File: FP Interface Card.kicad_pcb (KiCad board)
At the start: 6 copper layers, 90.2 x 101.1 mm, 274 parts, among them J1 T1M-10-F-SV-L, J2 T1M-10-F-SV-L, J3 ZX62-AB-5PA(31), J4 T1M-6-F-SV-L, J5 T1M-10-F-SV-L, P1 Card Edge for HSEC8-160-01-S-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, Q1 BC847BM3T5G, Q10 BSS138, Q11 BSS138, Q12 BSS138, Q13 BSS138DWQ-7, Q14 MMDT5551-7-F, Q15 BSS138DWQ-7, Q16 MMDT5551-7-F, Q17 MMBT4401-7-F, Q18 MMBT4401-7-F, Q19 IRF7404TRPBF, Q2 BC847BM3T5G, Q20 MMBT4401-7-F, Q21 IRF7404TRPBF, Q22 MMBT4401-7-F, Q23 IRF7404TRPBF, Q24 BSS138, Q25 BSS138, Q26 BSS138, Q27 BSS138, Q28 BSS138, Q3 BC847BM3T5G, Q4 BC847BM3T5G, Q5 BSS138DWQ-7, Q6 MMDT5551-7-F, Q7 BSS138DWQ-7, Q8 MMDT5551-7-F, Q9 BSS138, SW1 SW_Push_SPST, U1 DRV8838DSGT, U10 MAX7311AAG+, U11 MCP47FVB24-E/MQ, U12 ALM2402QPWPRQ1, U13 OPA340MDBVTEP, U14 AD7091R-5BCPZ-RL7, U15 ALM2402QPWPRQ1, U16 DRV8838DSGT, U17 INA240A3EDRQ1, U18 INA240A3EDRQ1, U19 DRV8838DSGT, U2 AP2161W, U20 INA240A3EDRQ1, U21 OPA340MDBVTEP, U22 OPA340MDBVTEP, U23 OPA340MDBVTEP, U24 RockBlock_9603, U3 IAM-20380, U4 IAM-20380, U5 PCA9543APW,118, U6 MMC5983MA, U7 MMC5983MA, U8 MXC6655XA, U9 MXC6655XA

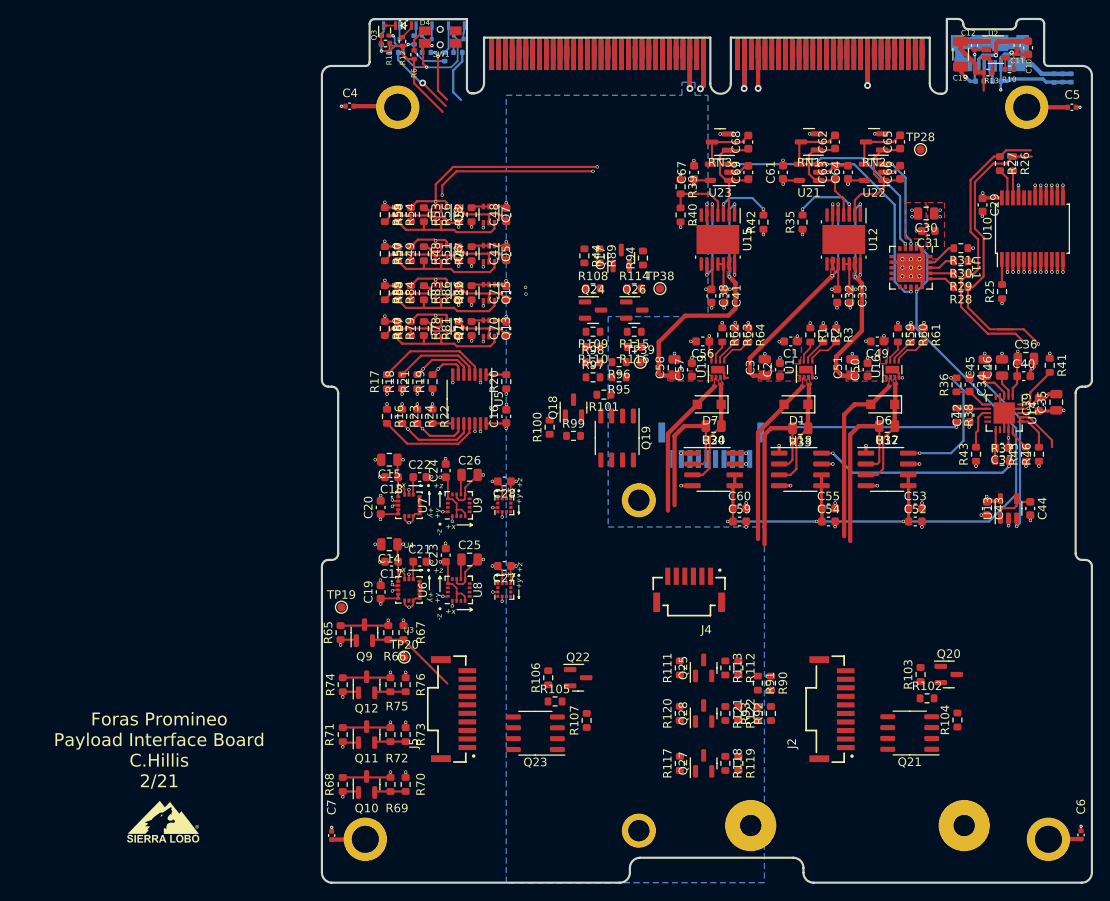
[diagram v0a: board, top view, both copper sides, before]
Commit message: friday changes
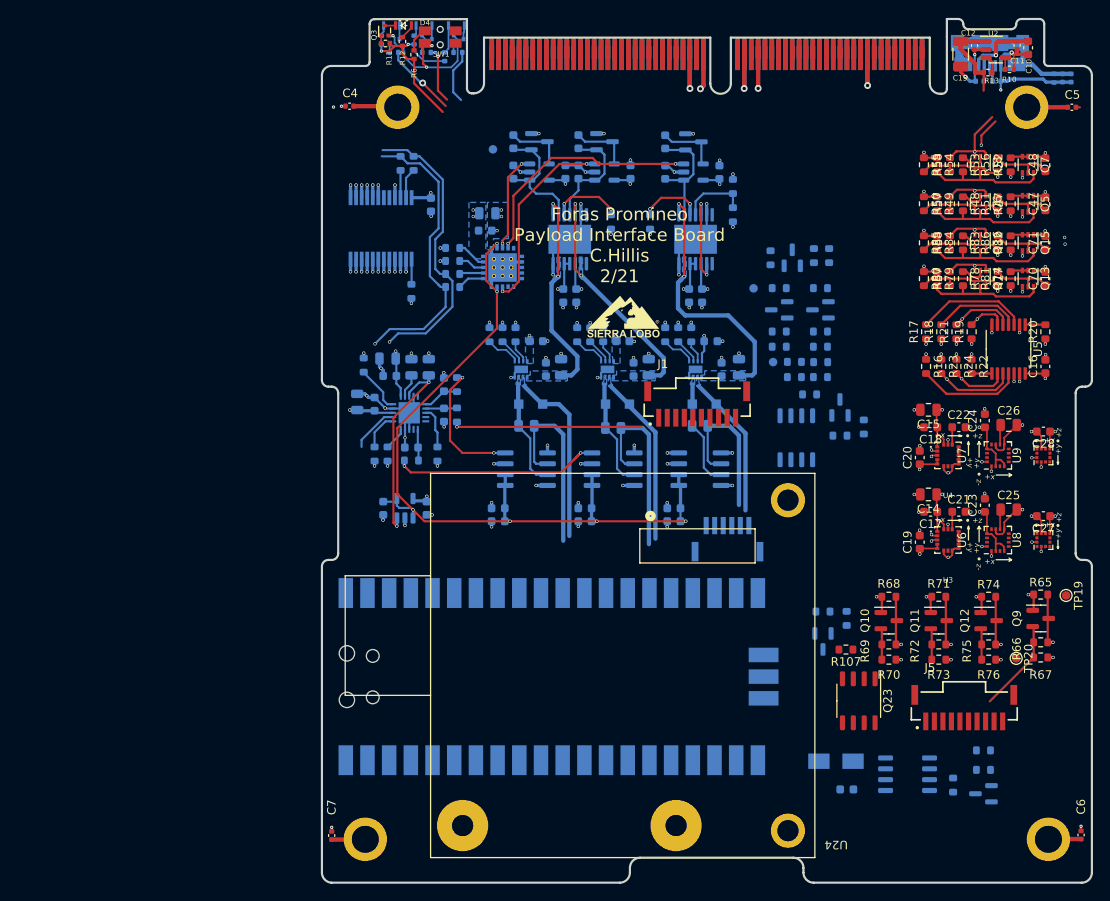
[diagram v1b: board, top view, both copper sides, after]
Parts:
- removed J2: T1M-10-F-SV-L, payload-interface-board:SAMTEC_T1M-10-F-SV-L
- removed Q25, Q27, Q28: BSS138, Package_TO_SOT_SMD:SOT-23
- removed R102: 100k, Resistor_SMD:R_0603_1608Metric
- removed R103, R111, R113, R117, R119, R120, R122: 10k, Resistor_SMD:R_0603_1608Metric
- removed R104: 3.3k, Resistor_SMD:R_0603_1608Metric
- removed R112, R118, R121: DNP, Resistor_SMD:R_0603_1608Metric
- removed R93: 0, Resistor_SMD:R_0603_1608Metric
- added C72: 1uF, Capacitor_SMD:C_0603_1608Metric, B.Cu at (61.5, -10.9)
- added D8: S1G, Diode_SMD:D_SMA, B.Cu at (60.2, -14.2)
- added U25: Pico, RPi_Pico:RPi_Pico_SMD_TH, B.Cu at (26.9, -24.1)
- C1, C2, C29, C3, C30, C31, C32, C33, C34, C35, C36, C37, C38, C39, C40, C41, C42, C43, C44, C45, C46, C49, C50, C51, C52, C53, C54, C55, C56, C57, C58, C59, C60, C61, C62, C63, C64, C65, C66, C67, C68, C69, D1, D6, D7, J4, Q17, Q18, Q19, Q20, Q21, Q22, Q24, Q26, R1, R100, R101, R105, R106, R108, R109, R110, R114, R115, R116, R2, R25, R26, R27, R28, R29, R3, R30, R31, R32, R33, R34, R35, R36, R37, R38, R39, R40, R41, R42, R43, R44, R45, R46, R59, R60, R61, R62, R63, R64, R89, R94, R95, R96, R97, R98, R99, RN1, RN2, RN3, TP28, TP38, TP39, U1, U10, U11, U12, U13, U14, U15, U16, U17, U18, U19, U20, U21, U22, U23: moved to B.Cu
- J1, U24: moved to F.Cu
- R90: value 0 -> 100k; moved to B.Cu
- R91: value 0 -> 10k; moved to B.Cu
- R92: value 0 -> 3.3k; moved to B.Cu
- moved TP19 84.9 mm to (87.1, -33.6), turned to -90 degrees
- moved R65 82.1 mm to (84.2, -33.7), turned to 0 degrees
- moved C35 81.9 mm to (4.13, -56.3)
- moved R41 80.3 mm to (4.89, -60.6)
- moved G*** 80.0 mm to (35.3, -66.3)
- moved Q9 79.2 mm to (84.2, -30.9), turned to 0 degrees
- moved C39 77.8 mm to (6.16, -56.0)
- moved R46 77.8 mm to (6.16, -50.2)
- moved R66 76.4 mm to (84.2, -28.1), turned to 180 degrees
- moved R74 76.3 mm to (78.1, -33.5), turned to 0 degrees
- moved U10 76.3 mm to (6.93, -76.6)
- moved C44 75.8 mm to (7.18, -43.9)
- moved C36 74.8 mm to (7.69, -61.4), turned to 180 degrees
- moved R45 74.8 mm to (7.69, -50.2)
- moved R67 74.7 mm to (84.2, -26.4), turned to 180 degrees
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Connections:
- net /ST_5V renamed Net-(C72-Pad1)
- Q20 pad 1: /PAYLOAD_PWR_SW -> /Pico/RB_PWR_SW_B
- R90 pad 1: /Level Shifter 7/io_hi -> /H2-22
- R90 pad 2: /ST_TXD -> GND
- R91 pad 1: /Level Shifter 7/io_hi -> /H2-22
- R91 pad 2: /ST_RXD -> /Pico/RB_PWR_SW_B
- R92 pad 1: /Level Shifter 8/io_hi -> +5V
- R92 pad 2: /ST_TXD -> Net-(Q20-Pad3)
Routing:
- net /H1-20: track 80.5 -> 12.7 mm
- net /H1-19: track 81.6 -> 14.7 mm
- net /H1-6: track 68.6 -> 5.98 mm
- net /H2-6: track 68.3 -> 6.40 mm
- net /SDA_SYS: track 42.9 -> 26.0 mm, vias 3 -> 2
- net /SCL_SYS: track 45.9 -> 29.9 mm, vias 4 -> 3
- net /RB_RxD: track 2.67 -> 0.00 mm, vias 2 -> 0
- net GND: track 191.4 -> 194.0 mm, vias 103 -> 105
- net /RB_Li-iON: track 1.34 -> 0.00 mm, vias 1 -> 0
- net /Magnetotorquer Drivers/Z_sen: track 22.2 -> 23.5 mm, vias 1 -> 2
- added copper zone on B.Cu, net +3V3
- added copper zone on B.Cu, net /Magnetotorquer Drivers/Full Bridge 1/OUT2
- added copper zone on B.Cu, net /Magnetotorquer Drivers/Full Bridge 2/OUT2
- added copper zone on B.Cu, net /Magnetotorquer Drivers/Full Bridge 3/OUT2
- added copper zone on B.Cu, net /Magnetotorquer Drivers/X_Drive
- added copper zone on B.Cu, net /Magnetotorquer Drivers/Y_Drive
- added copper zone on B.Cu, net /Magnetotorquer Drivers/Z_drive
- added copper zone on B.Cu, net /X+
- added copper zone on B.Cu, net /Y+
- added copper zone on B.Cu, net /Z+
- added copper zone on B.Cu, net GND
- removed copper zone on F.Cu, net +3V3
- removed copper zone on B.Cu, net +5V
- removed copper zone on F.Cu, net /Magnetotorquer Drivers/Full Bridge 1/OUT2
- removed copper zone on F.Cu, net /Magnetotorquer Drivers/Full Bridge 2/OUT2
- removed copper zone on F.Cu, net /Magnetotorquer Drivers/Full Bridge 3/OUT2
- removed copper zone on F.Cu, net /Magnetotorquer Drivers/X_Drive
- removed copper zone on F.Cu, net /Magnetotorquer Drivers/Y_Drive
- removed copper zone on F.Cu, net /Magnetotorquer Drivers/Z_drive
- removed copper zone on F.Cu, net /X+
- removed copper zone on F.Cu, net /Y+
- removed copper zone on F.Cu, net /Z+
- removed copper zone on F.Cu, net GND
